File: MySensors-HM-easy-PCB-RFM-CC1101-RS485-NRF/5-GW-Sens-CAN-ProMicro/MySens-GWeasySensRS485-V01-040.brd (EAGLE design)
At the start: 33 x 46 mm, 24 parts, among them IC1 ATSHA204A, IC2 LD117ADT50TR, IC6 LM1117MPX-ADJ, X4 1751264

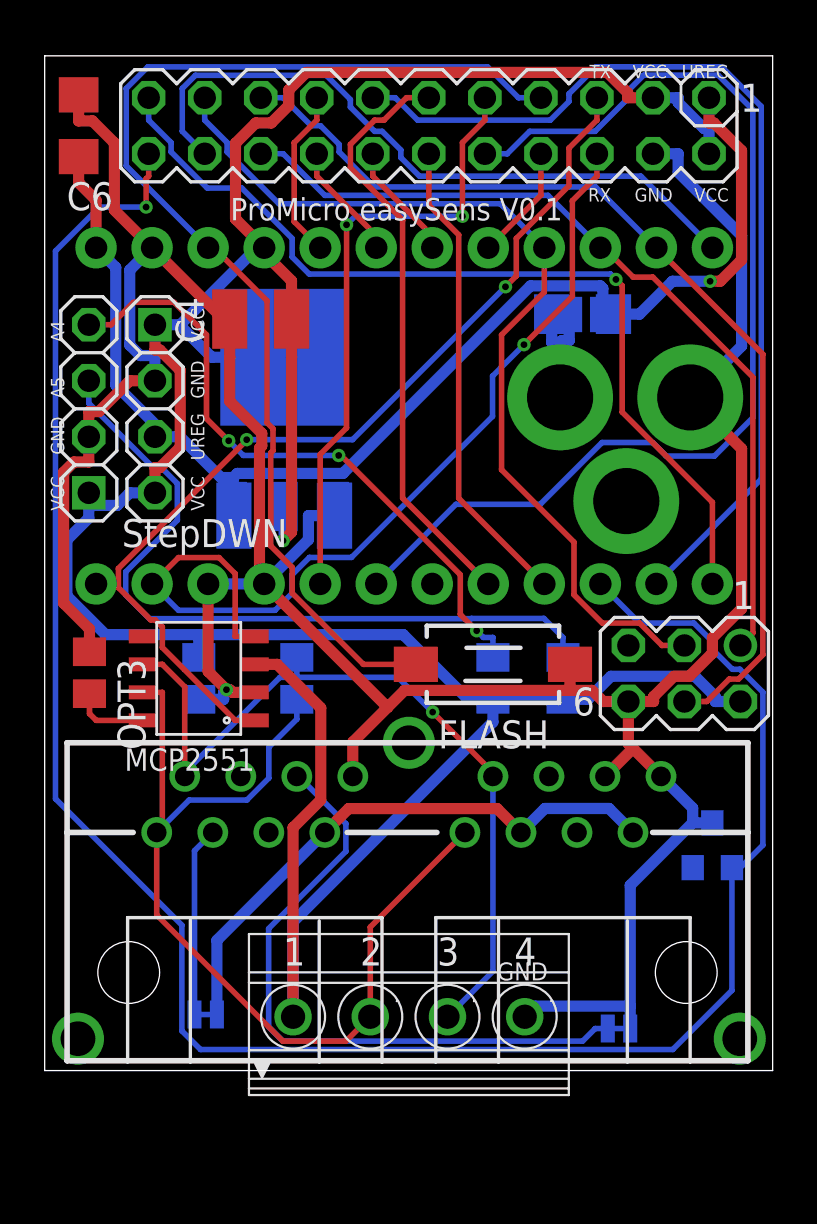
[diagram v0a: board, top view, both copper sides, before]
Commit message: Rework CAN
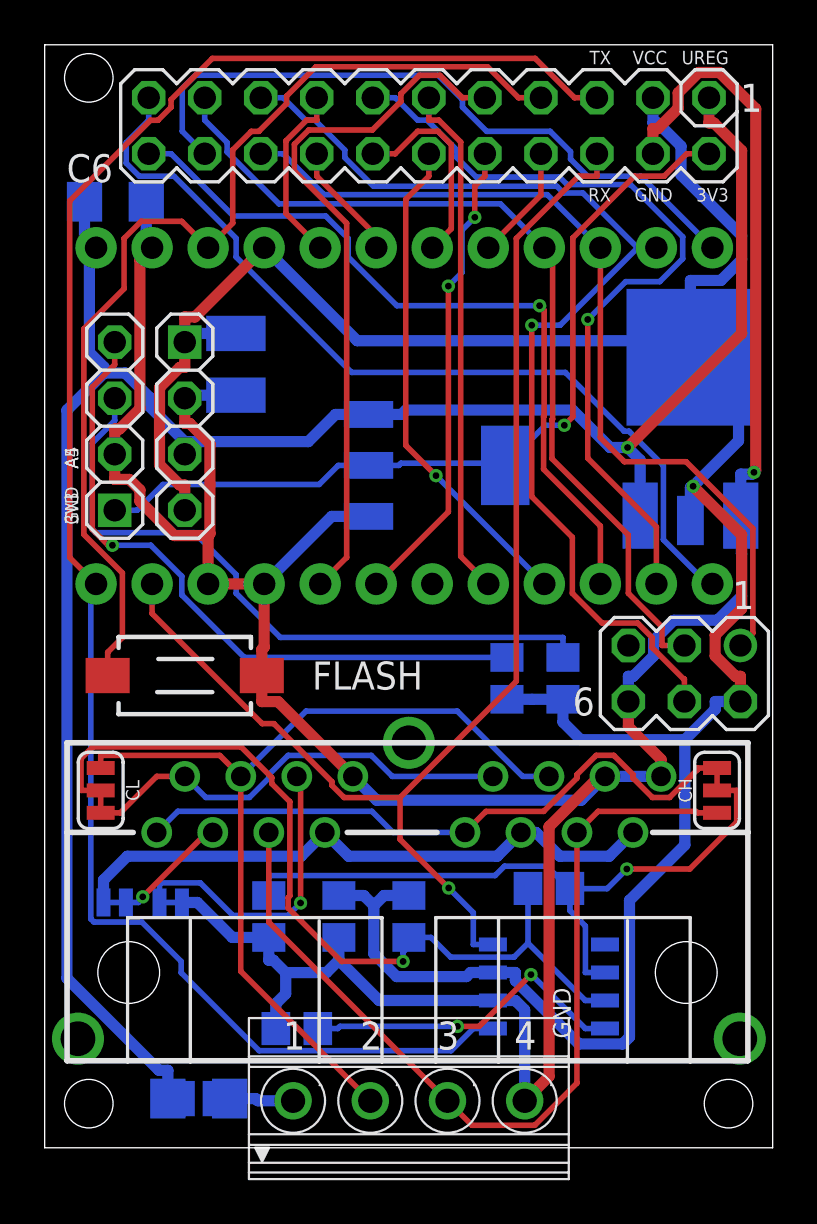
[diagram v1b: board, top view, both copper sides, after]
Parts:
- removed JP10: (no value), pinhead-2:1X04-S
- removed U$3: 2.1MMJACKTHM, adafruit:PJ-102A
- added CH, CL: JUMPER-SMT_3_1-NC_TRACE_SILK, SparkFun-Jumpers:SMT-JUMPER_3_1-NC_TRACE_SILK
- added I2C: (no value), pinhead-2:1X04-S
- added R3, R4: 680R, rcl:R0805
- IC1: value ATSHA204A -> LM1117MPX-ADJ; device Sensor:SOT23 -> lm1117:SOT223
- moved RAW1 39.6 mm to (6.99, -1.27), turned to 0 degrees
- moved F2 39.6 mm to (6.99, -1.27), turned to 180 degrees
- moved IC1 21.3 mm to (17.8, 27.4), turned to 90 degrees
- moved U$1 21.1 mm to (22.9, 3.81), flipped to the bottom
- moved JP3 21.1 mm to (5.71, 7.62)
- moved OPT3 18.7 mm to (11.4, 1.91), flipped to the bottom, turned to 180 degrees
- moved IC6 18.4 mm to (29.3, 28.0)
- moved IC2 18.4 mm to (29.3, 30.0)
- moved R6 14.9 mm to (22.9, 8.26), turned to 180 degrees
- moved FLASH 14.0 mm to (6.35, 17.9)
- moved C3 12.5 mm to (13.3, 6.99)
- moved JP1 6.54 mm to (3.17, 7.62), turned to 0 degrees
- moved C6 3.83 mm to (3.21, 39.4), flipped to the bottom, turned to 180 degrees
- moved X4 3.81 mm to (16.5, -1.27)
- moved C4 2.34 mm to (8.67, 32.0), flipped to the bottom, turned to 270 degrees
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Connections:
- removed net 4: J4.1-4
- removed net 5: J4.1-5
- removed net N$2: J4.2-4
- removed net N$3: J4.2-5
- new net CANH: CL.1, J4.1-4, J4.2-4, X4.2
- new net CANL: CH.1, J4.1-5, J4.2-5, X4.3
- new net H: CL.2, R3.2, R6.1, U$1.CANH
- new net L: CH.2, R4.1, R6.2, U$1.CANL
- net 3V3: now also I2C.1, IC1.TAB, SV2.2
- net A: now also CH.3; no longer R6.1, U$1.CANH, X4.2
- net A4: now also I2C.4; no longer JP10.4
- net A5: now also I2C.3; no longer JP10.3
- net B: now also CL.3; no longer R6.2, U$1.CANL, X4.3
- net D7: no longer IC1.1
- net GND: now also I2C.2, IC1.1, R4.2; no longer IC1.3, JP10.2, U$3.RING
- net UREG: now also IC1.3
- net VCC: now also R3.1; no longer JP10.1, SV2.2, X4.1
- net VIN: now also X4.1; no longer U$3.TIP
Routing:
- net D7: track 95.4 -> 34.8 mm
- net CANH: track 0.00 -> 40.9 mm
- net CANL: track 0.00 -> 40.8 mm
- net H: track 0.00 -> 38.7 mm, vias 0 -> 1
- net 3V3: track 0.00 -> 38.5 mm, vias 0 -> 1
- net TX1: track 44.2 -> 82.1 mm, vias 2 -> 0
- net UREG: track 57.4 -> 94.2 mm
- net L: track 0.00 -> 31.3 mm, vias 0 -> 1
- net D3: track 49.1 -> 21.5 mm, vias 0 -> 2
- net VCC: track 147.7 -> 123.0 mm
- net B: track 36.9 -> 20.1 mm, vias 1 -> 0
- net RX0: track 42.2 -> 58.4 mm
- net 2: track 29.7 -> 13.9 mm, vias 0 -> 1
- net A: track 43.9 -> 29.2 mm
- net RS: track 3.44 -> 15.0 mm, vias 0 -> 2
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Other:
- board size 33 x 46 mm -> 33 x 50 mm
- board text added: "3V3"
- board text added: "CANH"
- board text added: "CANL"
- board text added: "ProMicro easySens V0.2CAN"
- board text removed: "A"
- board text removed: "B"
- board text removed: "ProMicro easySens V0.1"
